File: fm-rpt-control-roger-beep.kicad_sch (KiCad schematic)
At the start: 21 parts, among them Q203 BC848, U201 HEF4093B, U202 74AHC1G32GW

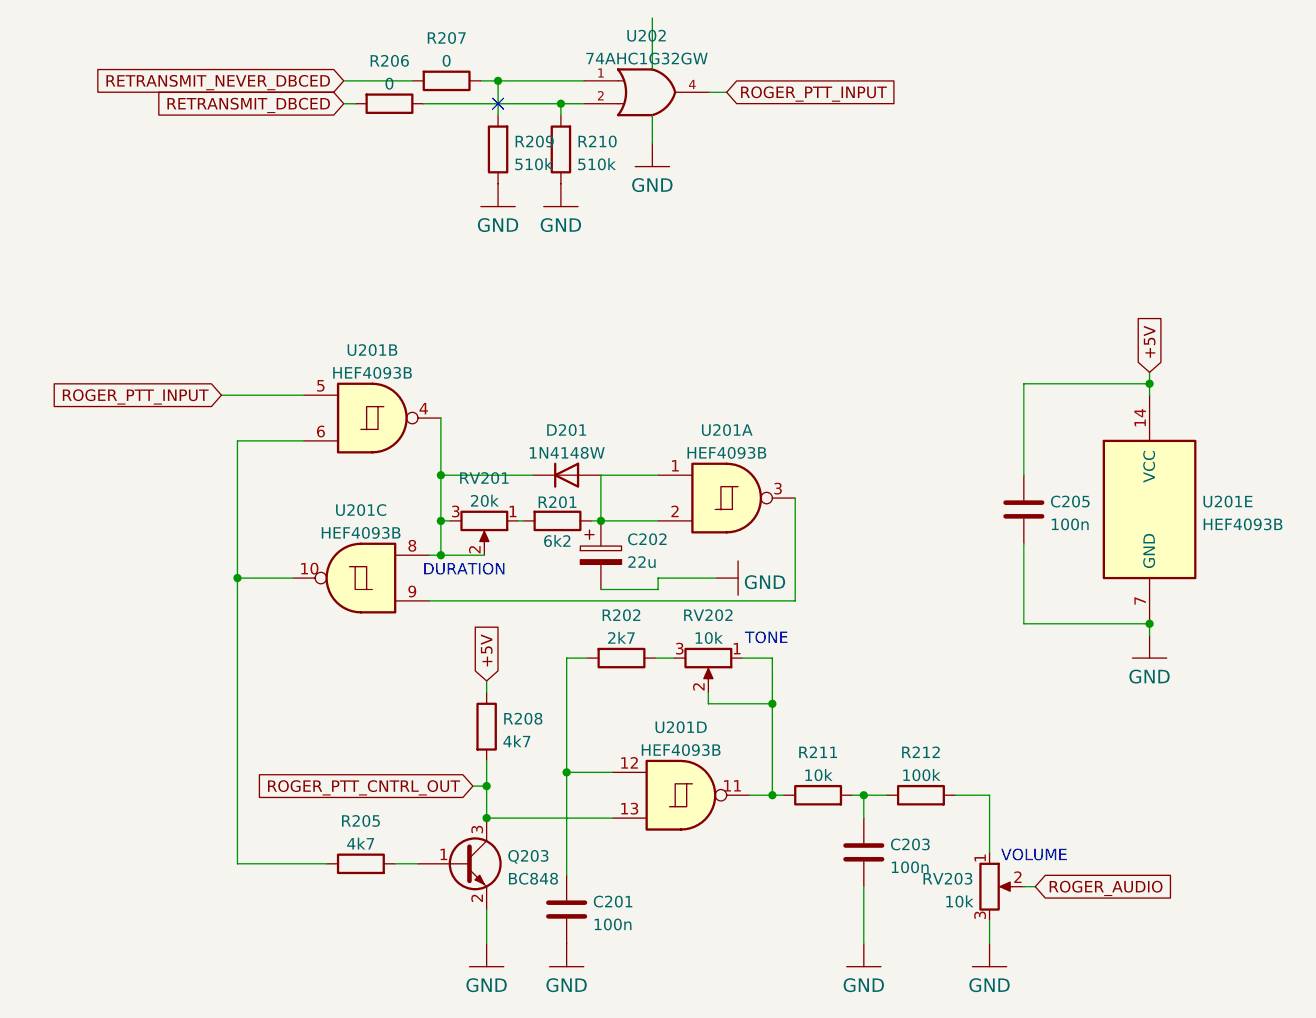
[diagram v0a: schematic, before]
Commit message: changing rogereep duration depends on simplex enable or not
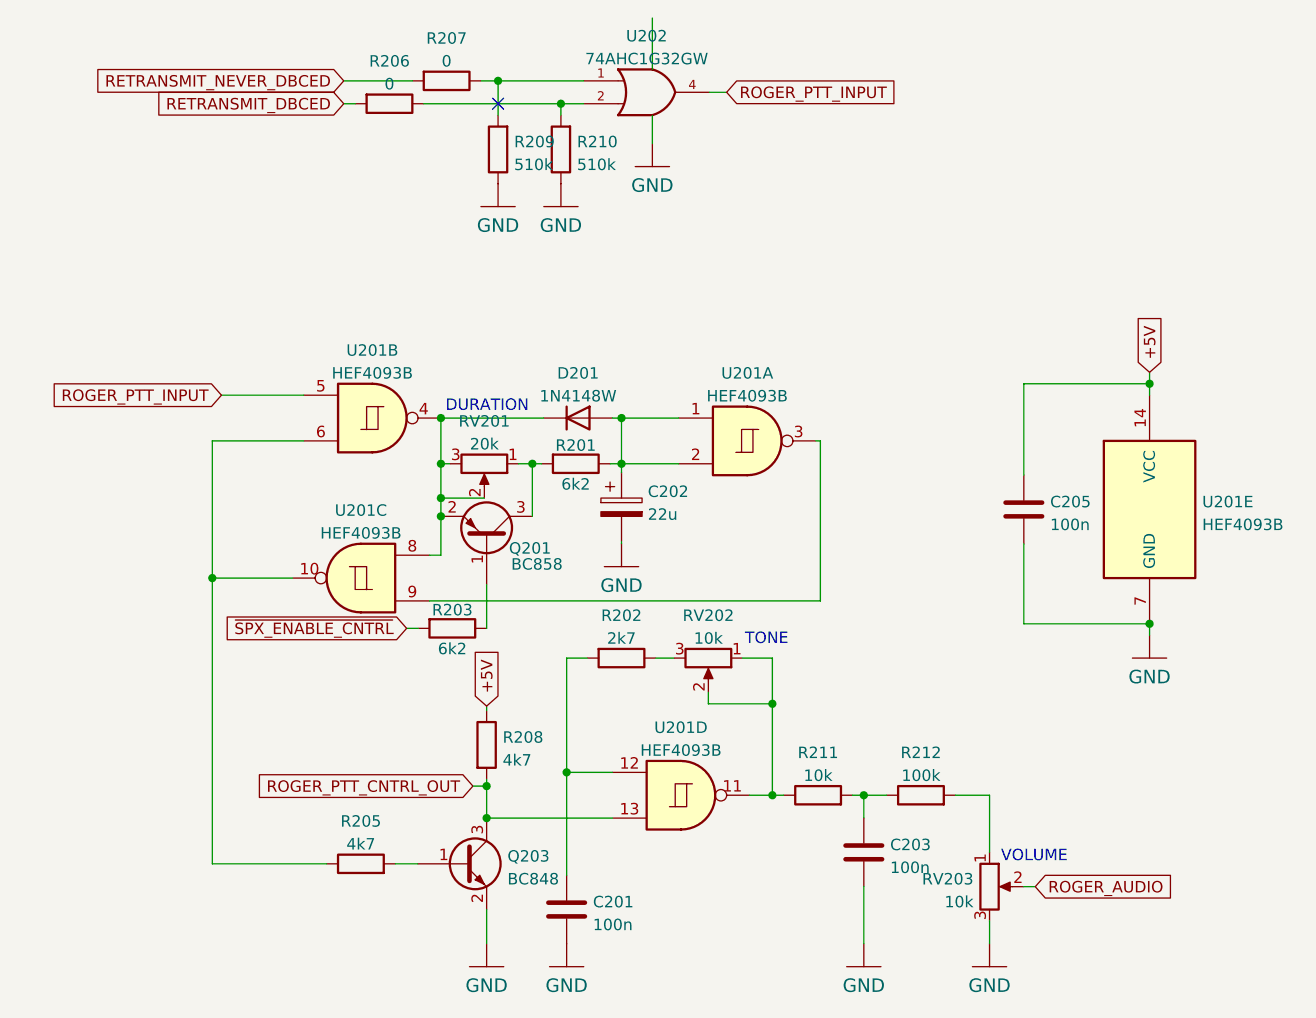
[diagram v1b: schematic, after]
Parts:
- added Q201: BC858, Package_TO_SOT_SMD:SOT-23, symbol Transistor_BJT:BC858
- added R203: 6k2, Resistor_SMD:R_0805_2012Metric_Pad1.20x1.40mm_HandSolder, symbol Device:R
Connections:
- net at R201.2, RV201.1: now also Q201.3 (C)
- net at D201.1 (K), RV201.2, RV201.3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: now also Q201.2 (E)
- new net: Q201.1 (B), R203.1
- new net ~{SPX_ENABLE_CNTRL}: R203.2
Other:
- moved on the sheet: C202, D201, R201, R208, RV201, U201A
